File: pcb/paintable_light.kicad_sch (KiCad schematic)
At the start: 19 parts, among them J2 Conn_01x02, J3 Conn_02x03_Odd_Even, U1 WS2811, U2 WS2811, U3 ATtiny85-20P

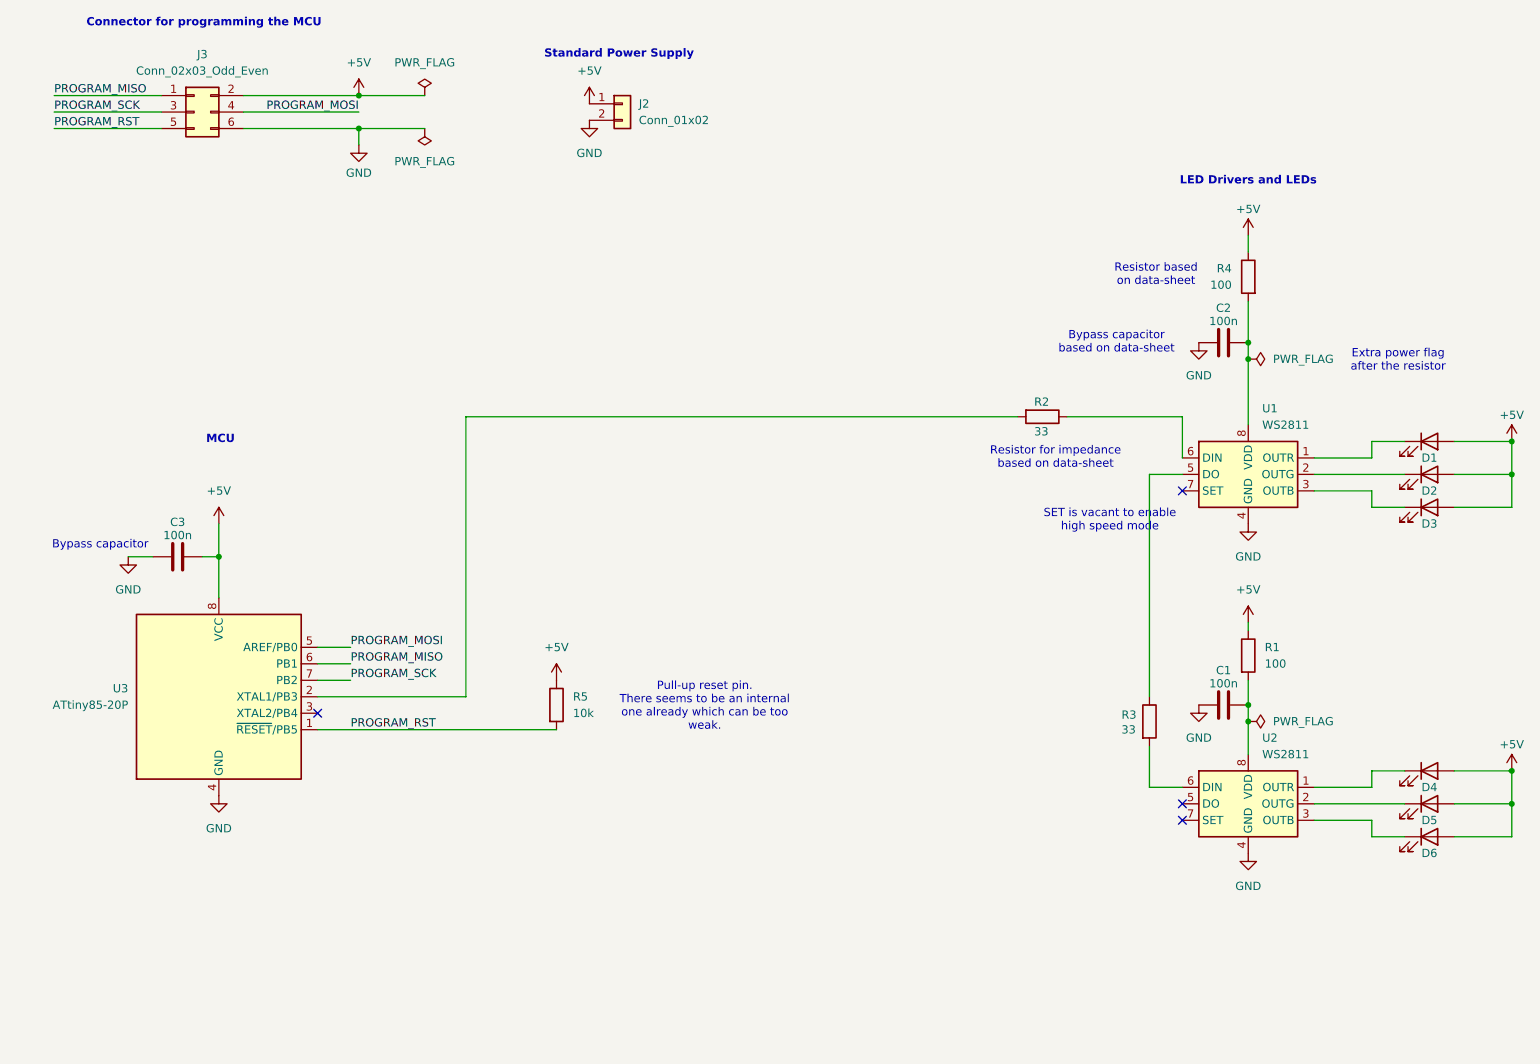
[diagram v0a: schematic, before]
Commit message: initial new board layout
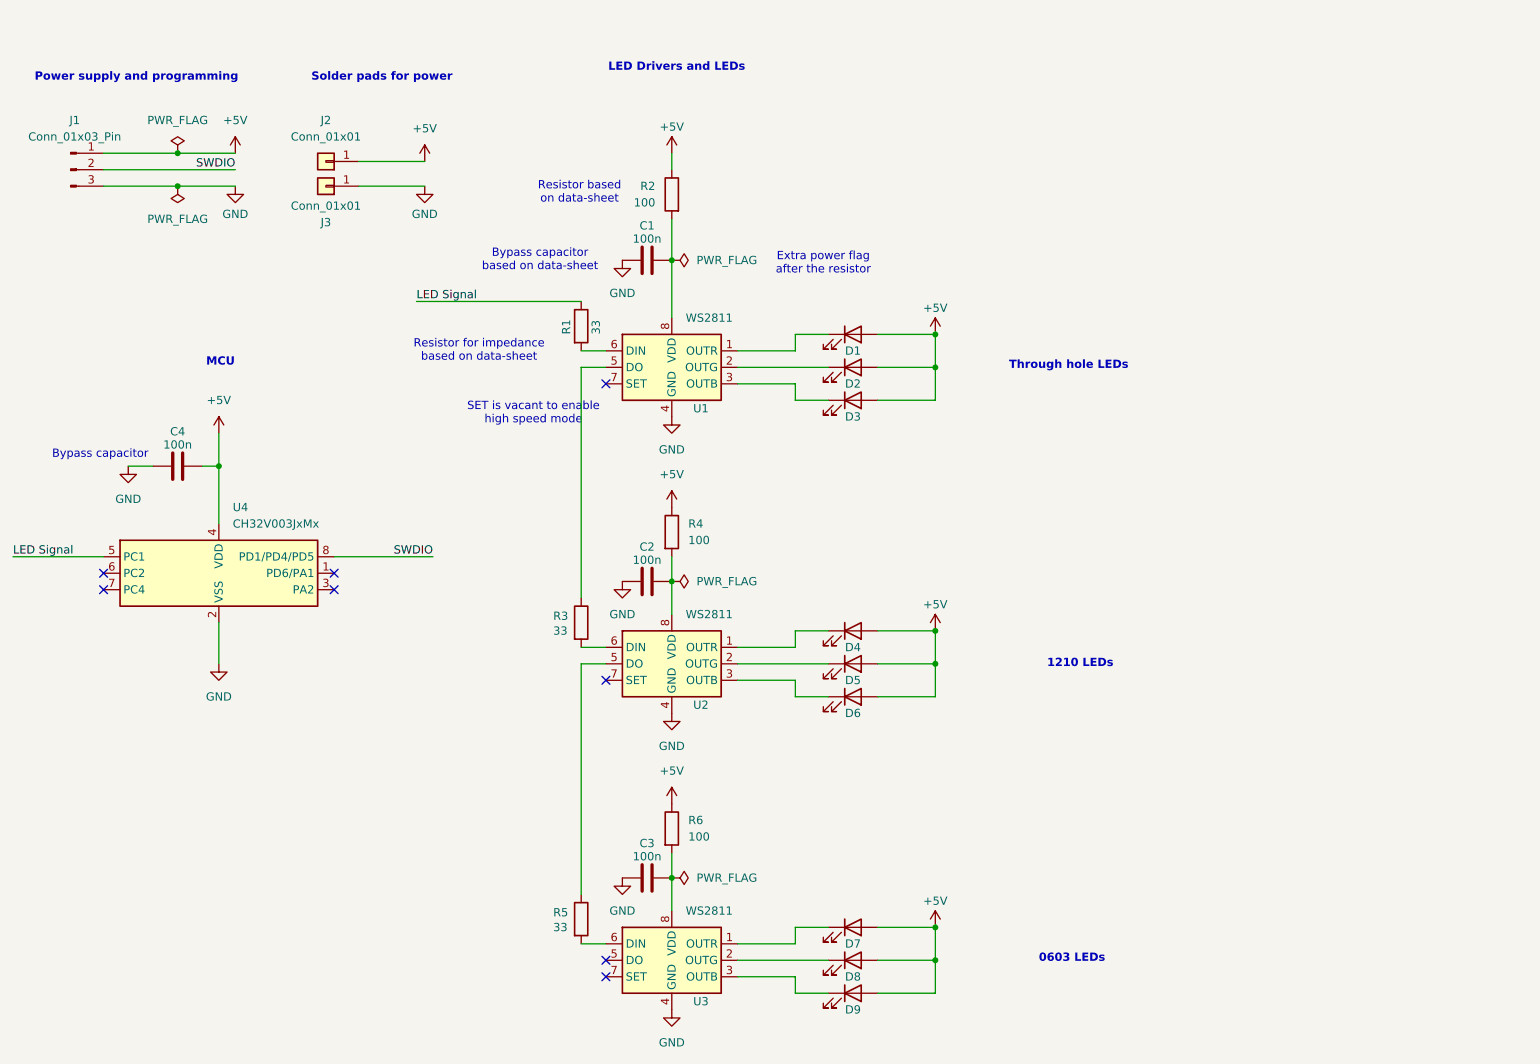
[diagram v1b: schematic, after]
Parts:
- removed J2: Conn_01x02, Connector_PinHeader_2.54mm:PinHeader_1x02_P2.54mm_Vertical, symbol Connector_Generic:Conn_01x02
- removed J3: Conn_02x03_Odd_Even, Connector_PinHeader_2.54mm:PinHeader_2x03_P2.54mm_Vertical, symbol Connector_Generic:Conn_02x03_Odd_Even
- removed U3: ATtiny85-20P, Package_DIP:DIP-8_W7.62mm, symbol MCU_Microchip_ATtiny:ATtiny85-20P
- added C3: 100n, Capacitor_SMD:C_1206_3216Metric_Pad1.33x1.80mm_HandSolder, symbol Device:C
- added D7, D8, D9: LED, LED_SMD:LED_0603_1608Metric_Pad1.05x0.95mm_HandSolder, symbol Device:LED
- added J1: Conn_01x03_Pin, Connector_PinHeader_2.54mm:PinHeader_1x03_P2.54mm_Vertical_SMD_Pin1Left, symbol Connector:Conn_01x03_Pin
- added J2, J3: Conn_01x01, TestPoint:TestPoint_Pad_2.5x2.5mm, symbol Connector_Generic:Conn_01x01
- added R6: 100, Resistor_SMD:R_1206_3216Metric_Pad1.30x1.75mm_HandSolder, symbol Device:R
- added U3: WS2811, Package_SO:SOIC-8_3.9x4.9mm_P1.27mm, symbol Driver_LED:WS2811
- added U4: CH32V003JxMx, Package_SO:JEITA_SOIC-8_3.9x4.9mm_P1.27mm, symbol MCU_WCH_RiscV:CH32V003JxMx
- C1: renamed from C2; footprint Capacitor_SMD:C_0603_1608Metric_Pad1.08x0.95mm_HandSolder -> Capacitor_SMD:C_1206_3216Metric_Pad1.33x1.80mm_HandSolder
- C2: renamed from C1; footprint Capacitor_SMD:C_0603_1608Metric_Pad1.08x0.95mm_HandSolder -> Capacitor_SMD:C_1206_3216Metric_Pad1.33x1.80mm_HandSolder
- C4: renamed from C3; footprint Capacitor_SMD:C_0603_1608Metric_Pad1.08x0.95mm_HandSolder -> Capacitor_SMD:C_1206_3216Metric_Pad1.33x1.80mm_HandSolder
- D1, D2, D3: footprint LED_SMD:LED_0603_1608Metric_Pad1.05x0.95mm_HandSolder -> LED_THT:LED_D5.0mm
- R1: renamed from R2; footprint Resistor_SMD:R_0603_1608Metric_Pad0.98x0.95mm_HandSolder -> Resistor_SMD:R_1206_3216Metric_Pad1.30x1.75mm_HandSolder
- R2: renamed from R4; footprint Resistor_SMD:R_0603_1608Metric_Pad0.98x0.95mm_HandSolder -> Resistor_SMD:R_1206_3216Metric_Pad1.30x1.75mm_HandSolder
- R3: footprint Resistor_SMD:R_0603_1608Metric_Pad0.98x0.95mm_HandSolder -> Resistor_SMD:R_1206_3216Metric_Pad1.30x1.75mm_HandSolder
- R4: renamed from R1; footprint Resistor_SMD:R_0603_1608Metric_Pad0.98x0.95mm_HandSolder -> Resistor_SMD:R_1206_3216Metric_Pad1.30x1.75mm_HandSolder
- R5: value 10k -> 33; footprint Resistor_SMD:R_0603_1608Metric_Pad0.98x0.95mm_HandSolder -> Resistor_SMD:R_1206_3216Metric_Pad1.30x1.75mm_HandSolder
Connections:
- net +5V: now also D7.2 (A), D8.2 (A), D9.2 (A), J1.1 (Pin_1), J2.1 (Pin_1), R6.1, U4.4 (VDD); no longer R5.1
- net GND: now also C3.1, J1.3 (Pin_3), J3.1 (Pin_1), U3.4 (GND), U4.2 (VSS)
- net at U1.6 (DIN): now also R1.2; no longer R1.1
- net at U2.5 (DO): now also R5.1
- net PROGRAM_RST: no longer names the net of R5.2
- net PROGRAM_RST: now also U3.6 (DIN)
- new net: D7.1 (K), U3.1 (OUTR)
- new net: D8.1 (K), U3.2 (OUTG)
- new net: D9.1 (K), U3.3 (OUTB)
- new net: C3.2, R6.2, U3.8 (VDD)
- new net LED Signal: R1.1, U4.5 (PC1)
- new net SWDIO: J1.2 (Pin_2), U4.8 (PD1/PD4/PD5)
- no-connect marks 4 -> 8
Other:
- note added: "0603 LEDs"
- note added: "1210 LEDs"
- note added: "Power supply and programming"
- note added: "Solder pads for power"
- note added: "Through hole LEDs"
- note removed: "Connector for programming the MCU"
- note removed: "Pull-up reset pin. There seems to be an internal one already which can be too weak."
- note removed: "Standard Power Supply"
- moved on the sheet: C1, C2, C4, D1, D2, D3, D4, D5, D6, R1, R2, R3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

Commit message: progress
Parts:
- D1, D2, D3: footprint LED_THT:LED_D5.0mm -> front_leds:LED_1210_3225Metric_Pad1.42x2.65mm_HandSolder_front
- D4, D5, D6: footprint LED_SMD:LED_1210_3225Metric_Pad1.42x2.65mm_HandSolder -> front_leds:LED_1210_3225Metric_Pad1.42x2.65mm_HandSolder_front
- D7, D8, D9: footprint LED_SMD:LED_0603_1608Metric_Pad1.05x0.95mm_HandSolder -> front_leds:LED_1210_3225Metric_Pad1.42x2.65mm_HandSolder_front
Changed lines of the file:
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@@
 			)
 		)
-		(property "Footprint" "LED_SMD:LED_0603_1608Metric_Pad1.05x0.95mm_HandSolder"
+		(property "Footprint" "front_leds:LED_1210_3225Metric_Pad1.42x2.65mm_HandSolder_front"
 			(at 156.21 157.48 0)
 			(effects
@@
 			)
 		)
-		(property "Footprint" "LED_SMD:LED_1210_3225Metric_Pad1.42x2.65mm_HandSolder"
+		(property "Footprint" "front_leds:LED_1210_3225Metric_Pad1.42x2.65mm_HandSolder_front"
 			(at 156.21 116.84 0)
 			(effects
@@
 			)
 		)
-		(property "Footprint" "LED_THT:LED_D5.0mm"
+		(property "Footprint" "front_leds:LED_1210_3225Metric_Pad1.42x2.65mm_HandSolder_front"
 			(at 156.21 66.04 0)
 			(effects
@@
 			)
 		)
-		(property "Footprint" "LED_THT:LED_D5.0mm"
+		(property "Footprint" "front_leds:LED_1210_3225Metric_Pad1.42x2.65mm_HandSolder_front"
 			(at 156.21 71.12 0)
 			(effects
@@
 			)
 		)
-		(property "Footprint" "LED_THT:LED_D5.0mm"
+		(property "Footprint" "front_leds:LED_1210_3225Metric_Pad1.42x2.65mm_HandSolder_front"
 			(at 156.21 76.2 0)
 			(effects
@@
 			)
 		)
-		(property "Footprint" "LED_SMD:LED_1210_3225Metric_Pad1.42x2.65mm_HandSolder"
+		(property "Footprint" "front_leds:LED_1210_3225Metric_Pad1.42x2.65mm_HandSolder_front"
 			(at 156.21 111.76 0)
 			(effects
@@
 			)
 		)
-		(property "Footprint" "LED_SMD:LED_0603_1608Metric_Pad1.05x0.95mm_HandSolder"
+		(property "Footprint" "front_leds:LED_1210_3225Metric_Pad1.42x2.65mm_HandSolder_front"
 			(at 156.21 167.64 0)
 			(effects
@@
 			)
 		)
-		(property "Footprint" "LED_SMD:LED_0603_1608Metric_Pad1.05x0.95mm_HandSolder"
+		(property "Footprint" "front_leds:LED_1210_3225Metric_Pad1.42x2.65mm_HandSolder_front"
 			(at 156.21 162.56 0)
 			(effects
@@
 			)
 		)
-		(property "Footprint" "LED_SMD:LED_1210_3225Metric_Pad1.42x2.65mm_HandSolder"
+		(property "Footprint" "front_leds:LED_1210_3225Metric_Pad1.42x2.65mm_HandSolder_front"
 			(at 156.21 121.92 0)
 			(effects
